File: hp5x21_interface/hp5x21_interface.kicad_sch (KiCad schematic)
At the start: 4 parts, among them IC1 74LVC4245APW,118, IC2 74LVC4245APW,118, IC3 74LVC4245APW,118

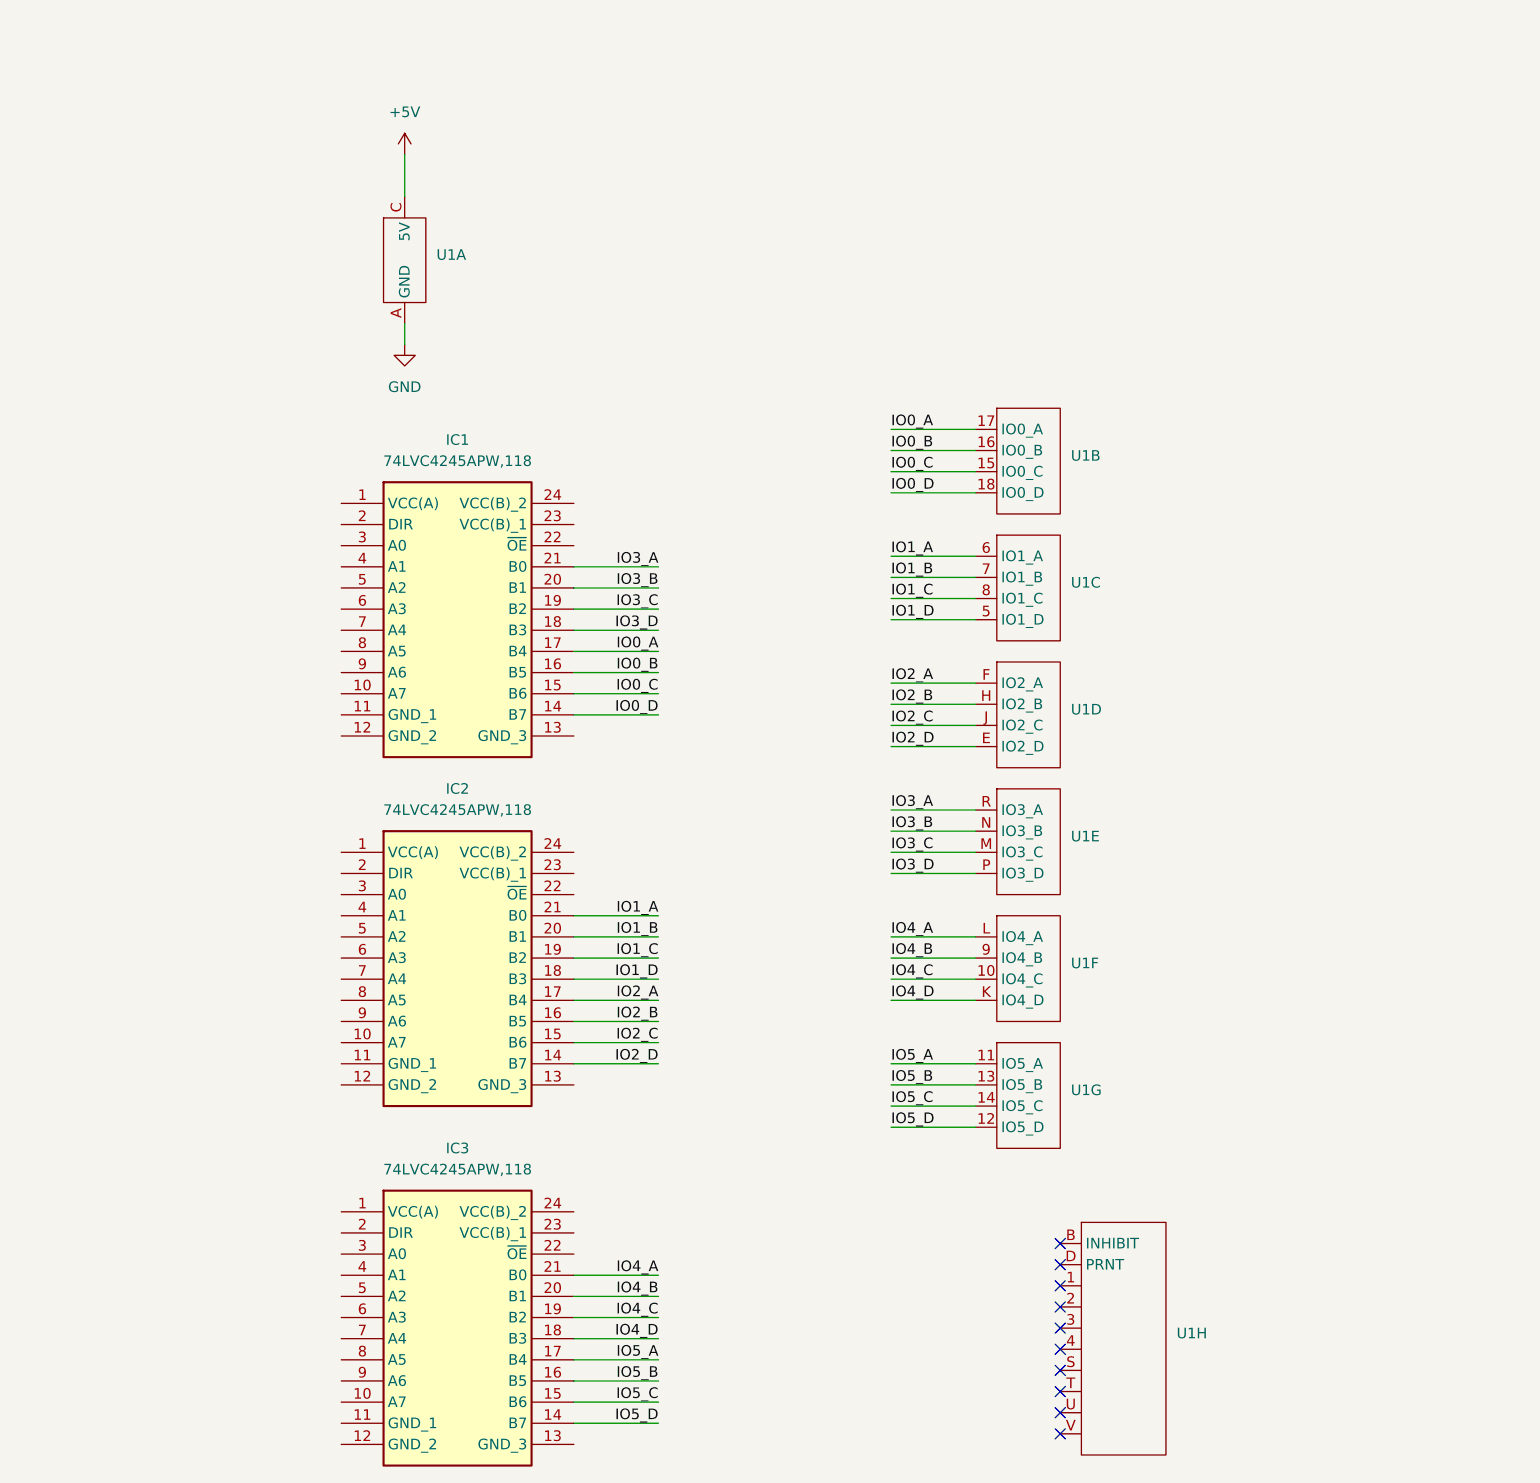
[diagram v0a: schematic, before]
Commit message: Updated and released to JLCPCB
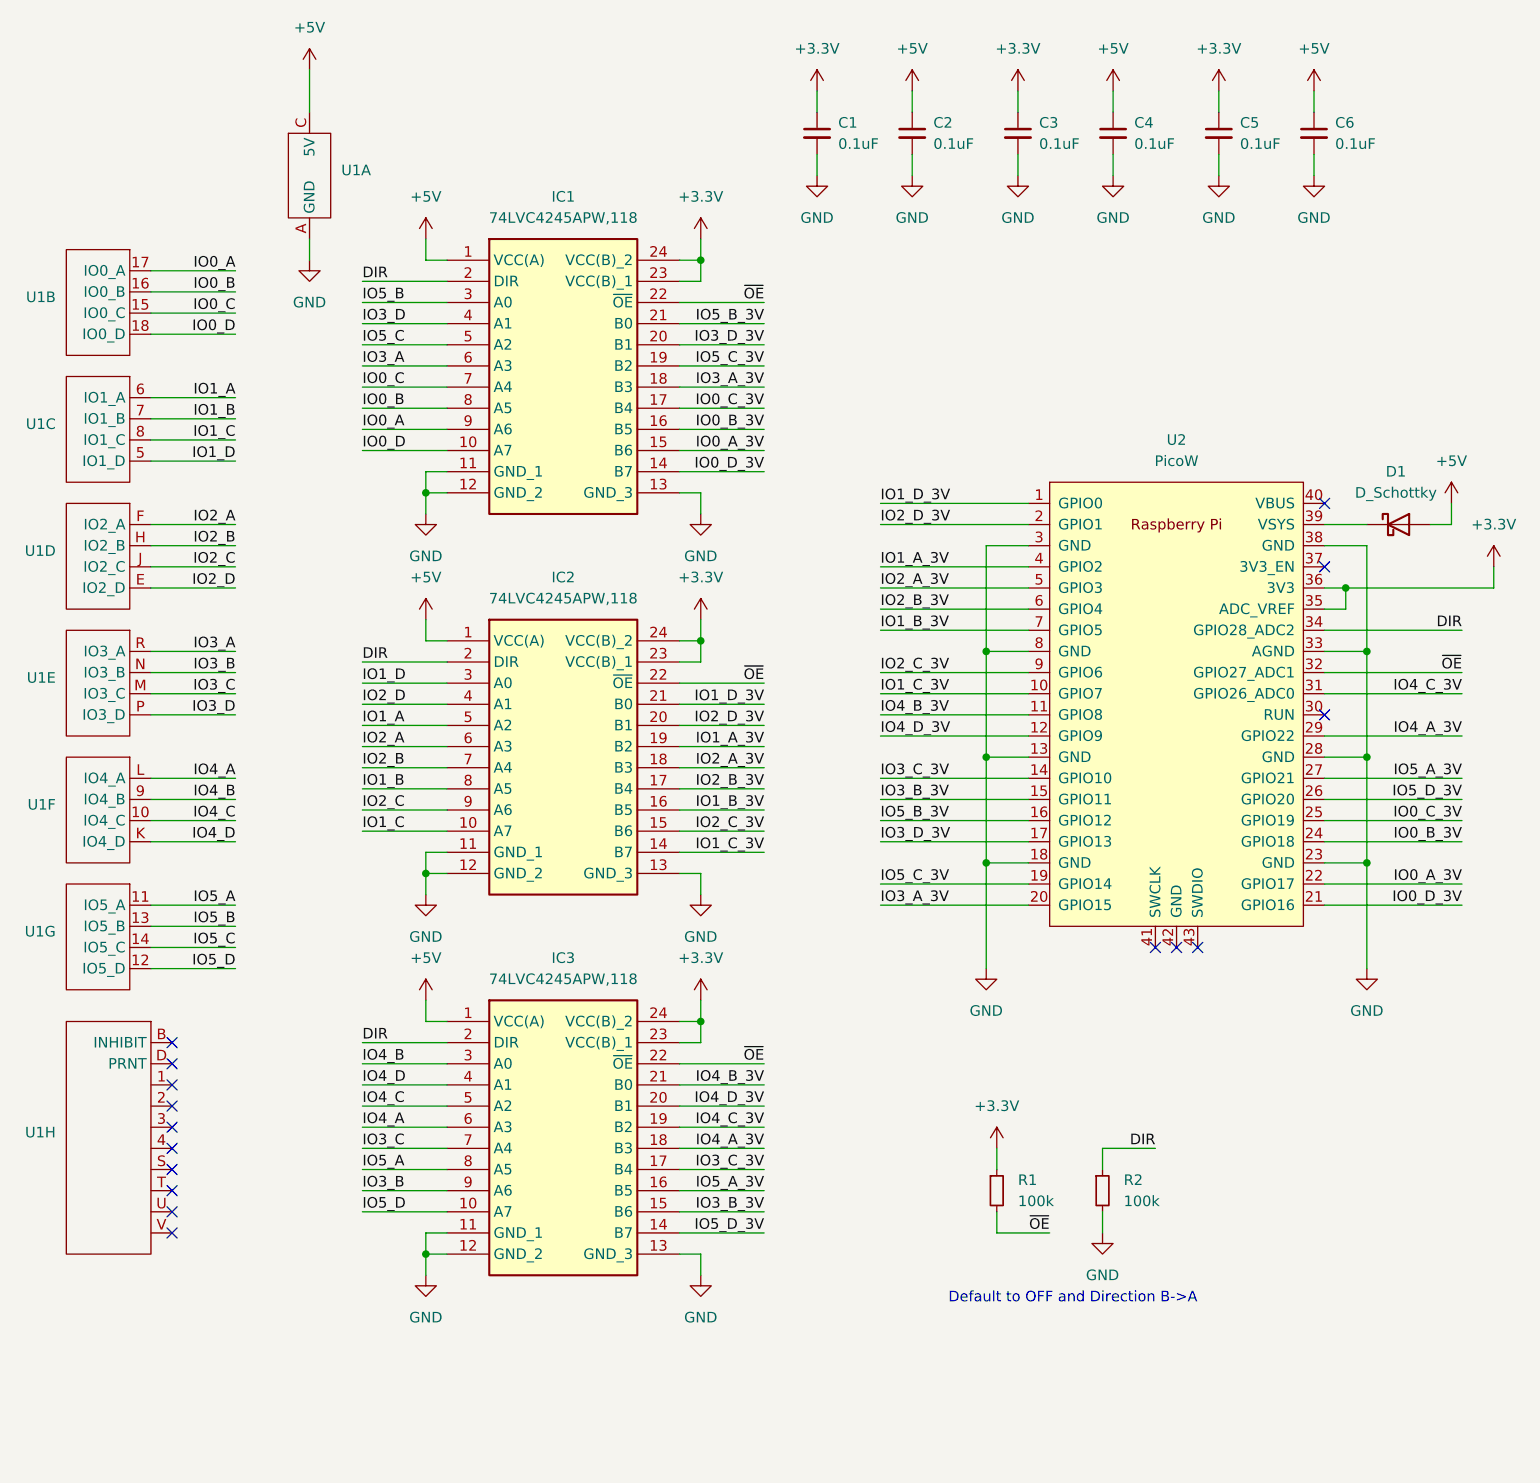
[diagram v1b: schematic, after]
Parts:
- added C1, C2, C3, C4, C5, C6: 0.1uF, Capacitor_SMD:C_0402_1005Metric, symbol Device:C_Small
- added D1: D_Schottky, Diode_SMD:D_SOD-123, symbol Device:D_Schottky
- added R1, R2: 100k, Resistor_SMD:R_0402_1005Metric, symbol Device:R_Small
- added U2: PicoW, RP2040:RPi_PicoW_SMD_TH, symbol RP2040:PicoW
- U1: value ~ -> 307-036-520-201
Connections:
- net +5V: now also IC1.1 (VCC(A)), IC2.1 (VCC(A)), IC3.1 (VCC(A)), C2.1, C4.1, C6.1, D1.2 (A)
- net GND: now also IC1.11 (GND_1), IC1.12 (GND_2), IC1.13 (GND_3), IC2.11 (GND_1), IC2.12 (GND_2), IC2.13 (GND_3), IC3.11 (GND_1), IC3.12 (GND_2), IC3.13 (GND_3), C1.2, C2.2, C3.2, C4.2, C5.2, C6.2, R2.2, U2.13 (GND), U2.18 (GND), U2.23 (GND), U2.28 (GND), U2.3 (GND), U2.33 (AGND), U2.38 (GND), U2.8 (GND)
- net IO0_A: now also IC1.9 (A6); no longer IC1.17 (B4)
- net IO0_B: now also IC1.8 (A5); no longer IC1.16 (B5)
- net IO0_C: now also IC1.7 (A4); no longer IC1.15 (B6)
- net IO0_D: now also IC1.10 (A7); no longer IC1.14 (B7)
- net IO1_A: now also IC2.5 (A2); no longer IC2.21 (B0)
- net IO1_B: now also IC2.8 (A5); no longer IC2.20 (B1)
- net IO1_C: now also IC2.10 (A7); no longer IC2.19 (B2)
- net IO1_D: now also IC2.3 (A0); no longer IC2.18 (B3)
- net IO2_A: now also IC2.6 (A3); no longer IC2.17 (B4)
- net IO2_B: now also IC2.7 (A4); no longer IC2.16 (B5)
- net IO2_C: now also IC2.9 (A6); no longer IC2.15 (B6)
- net IO2_D: now also IC2.4 (A1); no longer IC2.14 (B7)
- net IO3_A: now also IC1.6 (A3); no longer IC1.21 (B0)
- net IO3_B: now also IC3.9 (A6); no longer IC1.20 (B1)
- net IO3_C: now also IC3.7 (A4); no longer IC1.19 (B2)
- net IO3_D: now also IC1.4 (A1); no longer IC1.18 (B3)
- net IO4_A: now also IC3.6 (A3); no longer IC3.21 (B0)
- net IO4_B: now also IC3.3 (A0); no longer IC3.20 (B1)
- net IO4_C: now also IC3.5 (A2); no longer IC3.19 (B2)
- net IO4_D: now also IC3.4 (A1); no longer IC3.18 (B3)
- net IO5_A: now also IC3.8 (A5); no longer IC3.17 (B4)
- net IO5_B: now also IC1.3 (A0); no longer IC3.16 (B5)
- net IO5_C: now also IC1.5 (A2); no longer IC3.15 (B6)
- net IO5_D: now also IC3.10 (A7); no longer IC3.14 (B7)
- net DIR: now reaches IC2.2 (DIR)
- net DIR: now also IC1.2 (DIR), IC3.2 (DIR), R2.1, U2.34 (GPIO28_ADC2)
- net ~{OE}: now reaches IC2.22 (~{OE})
- net ~{OE}: now also IC1.22 (~{OE}), IC3.22 (~{OE}), R1.2, U2.32 (GPIO27_ADC1)
- net +3.3V: now reaches IC2.23 (VCC(B)_1)
- net +3.3V: now also IC1.23 (VCC(B)_1), IC1.24 (VCC(B)_2), IC2.24 (VCC(B)_2), IC3.23 (VCC(B)_1), IC3.24 (VCC(B)_2), C1.1, C3.1, C5.1, R1.1, U2.35 (ADC_VREF), U2.36 (3V3)
- new net: D1.1 (K), U2.39 (VSYS)
- new net IO0_A_3V: IC1.15 (B6), U2.22 (GPIO17)
- new net IO0_B_3V: IC1.16 (B5), U2.24 (GPIO18)
- new net IO0_C_3V: IC1.17 (B4), U2.25 (GPIO19)
- new net IO0_D_3V: IC1.14 (B7), U2.21 (GPIO16)
- new net IO1_A_3V: IC2.19 (B2), U2.4 (GPIO2)
- new net IO1_B_3V: IC2.16 (B5), U2.7 (GPIO5)
- new net IO1_C_3V: IC2.14 (B7), U2.10 (GPIO7)
- new net IO1_D_3V: IC2.21 (B0), U2.1 (GPIO0)
- new net IO2_A_3V: IC2.18 (B3), U2.5 (GPIO3)
- new net IO2_B_3V: IC2.17 (B4), U2.6 (GPIO4)
- new net IO2_C_3V: IC2.15 (B6), U2.9 (GPIO6)
- new net IO2_D_3V: IC2.20 (B1), U2.2 (GPIO1)
- new net IO3_A_3V: IC1.18 (B3), U2.20 (GPIO15)
- new net IO3_B_3V: IC3.15 (B6), U2.15 (GPIO11)
- new net IO3_C_3V: IC3.17 (B4), U2.14 (GPIO10)
- new net IO3_D_3V: IC1.20 (B1), U2.17 (GPIO13)
- new net IO4_A_3V: IC3.18 (B3), U2.29 (GPIO22)
- new net IO4_B_3V: IC3.21 (B0), U2.11 (GPIO8)
- new net IO4_C_3V: IC3.19 (B2), U2.31 (GPIO26_ADC0)
- new net IO4_D_3V: IC3.20 (B1), U2.12 (GPIO9)
- new net IO5_A_3V: IC3.16 (B5), U2.27 (GPIO21)
- new net IO5_B_3V: IC1.21 (B0), U2.16 (GPIO12)
- new net IO5_C_3V: IC1.19 (B2), U2.19 (GPIO14)
- new net IO5_D_3V: IC3.14 (B7), U2.26 (GPIO20)
- no-connect marks 10 -> 16
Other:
- note added: "Default to OFF and Direction B->A"
- company: (none) -> alvarop.com
- title: (none) -> HP 5x21 Interface (RPi Pico W Edition)
- moved on the sheet: IC1, IC2, IC3, U1A, U1B, U1C, U1D, U1E, U1F, U1G, U1H
